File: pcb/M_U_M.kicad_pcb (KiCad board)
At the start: 2 copper layers, 28 parts, among them J1 Conn_01x04, SW1 RotaryEncoder_Switch, SW10 SW_Push, SW11 SW_Push, SW12 SW_Push, SW2 RotaryEncoder_Switch, SW3 SW_Push, SW4 SW_Push, SW5 SW_Push, SW6 SW_Push, SW7 SW_Push, SW8 SW_Push, SW9 SW_Push, U1 RP2040-ZERO

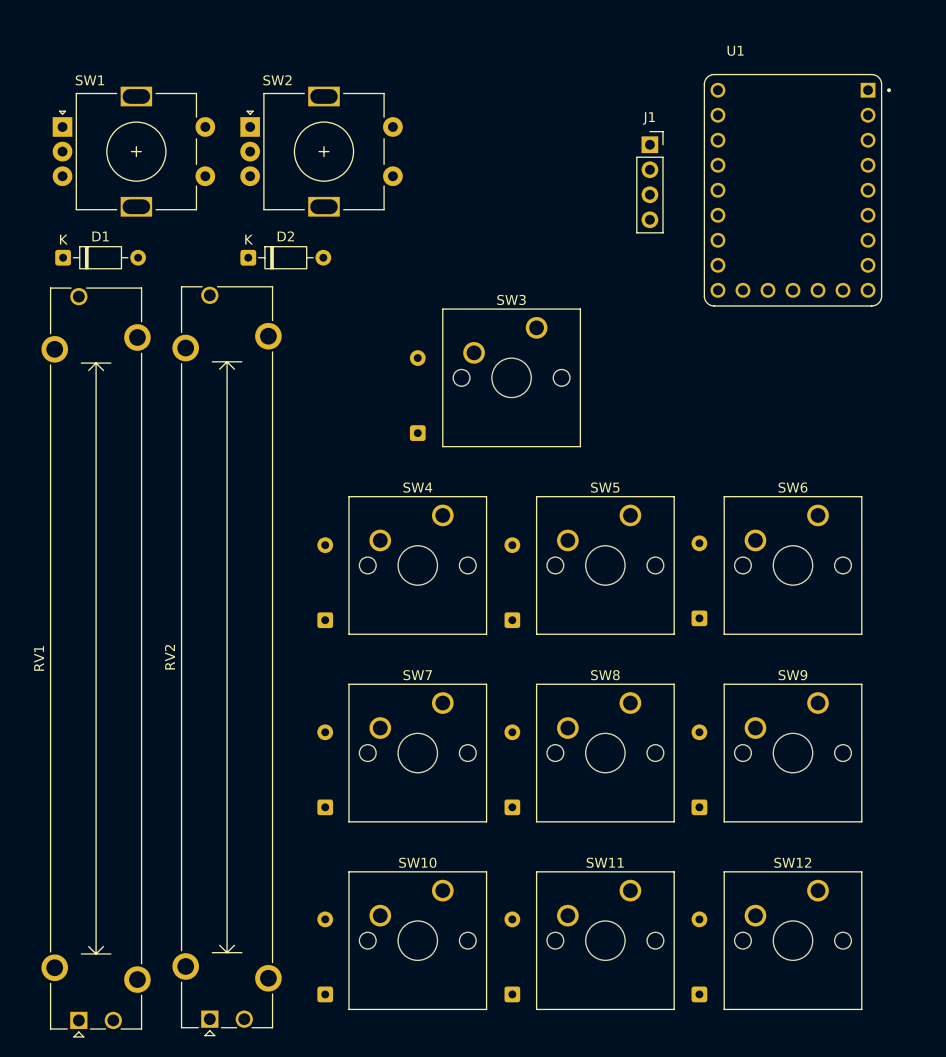
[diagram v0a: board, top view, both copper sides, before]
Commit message: we updated and routed
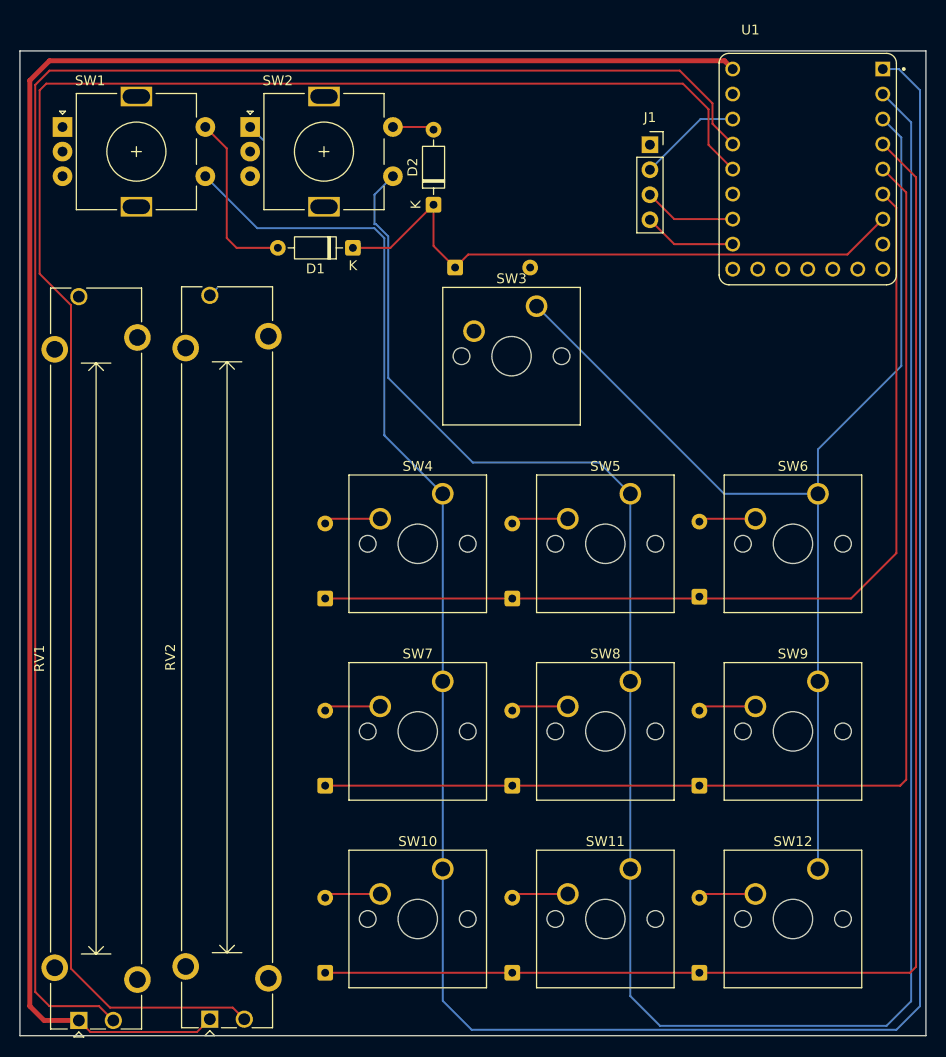
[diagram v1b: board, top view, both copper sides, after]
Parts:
- moved D1 29.4 mm to (145.8, 63.0), turned to 180 degrees
- moved D2 19.6 mm to (154.0, 58.6), turned to 90 degrees
- moved D3 17.2 mm to (156.2, 65.0), turned to 0 degrees
- moved U1 2.62 mm to (192.0, 55.0)
- moved SW10 2.20 mm to (154.9, 126.1)
- moved SW11 2.20 mm to (174.0, 126.1)
- moved SW12 2.20 mm to (193.0, 126.1)
- moved D4 2.20 mm to (143.0, 98.6)
- moved D5 2.20 mm to (162.0, 98.6)
- moved D6 2.20 mm to (181.0, 98.4)
- moved D7 2.20 mm to (143.0, 117.6)
- moved D8 2.20 mm to (162.0, 117.6)
- moved D9 2.20 mm to (181.0, 117.6)
- moved SW3 2.20 mm to (164.5, 68.9)
- moved SW4 2.20 mm to (154.9, 88.0)
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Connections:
- U1 pad 12: unconnected-(U1-GP11-Pad12) -> /R1A
- U1 pad 13: /R1A -> /R1B
- U1 pad 14: /R1B -> /R2A
- U1 pad 15: /R2A -> /R2B
- U1 pad 16: /R2B -> /SDA
- U1 pad 17: unconnected-(U1-GP26-Pad17) -> /SCL
- U1 pad 19: /POT1 -> /POT2
- U1 pad 20: /POT2 -> /POT1
- U1 pad 4: /ROW0 -> /ROW3
- U1 pad 5: /ROW1 -> /ROW2
- U1 pad 6: /ROW2 -> /ROW1
- U1 pad 7: /ROW3 -> /ROW0
- U1 pad 8: /SCL -> unconnected-(U1-GP7-Pad8)
- U1 pad 9: /SDA -> unconnected-(U1-GP8-Pad9)
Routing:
- net /COL0: track 0.00 -> 249.0 mm
- net /COL1: track 0.00 -> 226.5 mm
- net /POT2: track 0.00 -> 186.6 mm
- net +5V: track 0.00 -> 186.5 mm
- net /POT1: track 0.00 -> 177.0 mm
- net /ROW3: track 0.00 -> 145.2 mm
- net /ROW2: track 0.00 -> 122.2 mm
- net /COL2: track 0.00 -> 116.9 mm
- net /ROW1: track 0.00 -> 96.9 mm
- net /ROW0: track 0.00 -> 63.4 mm
- net /R1S2: track 0.00 -> 17.8 mm
- net +3V3: track 0.00 -> 10.5 mm
- net /SDA: track 0.00 -> 9.43 mm
- net /SCL: track 0.00 -> 9.43 mm
- net Net-(D9-A): track 0.00 -> 5.87 mm
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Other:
- board outline added: 92 x 100 mm
